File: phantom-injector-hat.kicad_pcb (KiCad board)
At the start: 2 copper layers, 65 x 44.8 mm, 42 parts, among them J1 Conn_02x20_Odd_Even, J2 Conn_02x03_Top_Bottom, J3 Conn_01x03, J4 Conn_01x03, SW1 SW_SPST, U1 LT8362EMSE-PBF

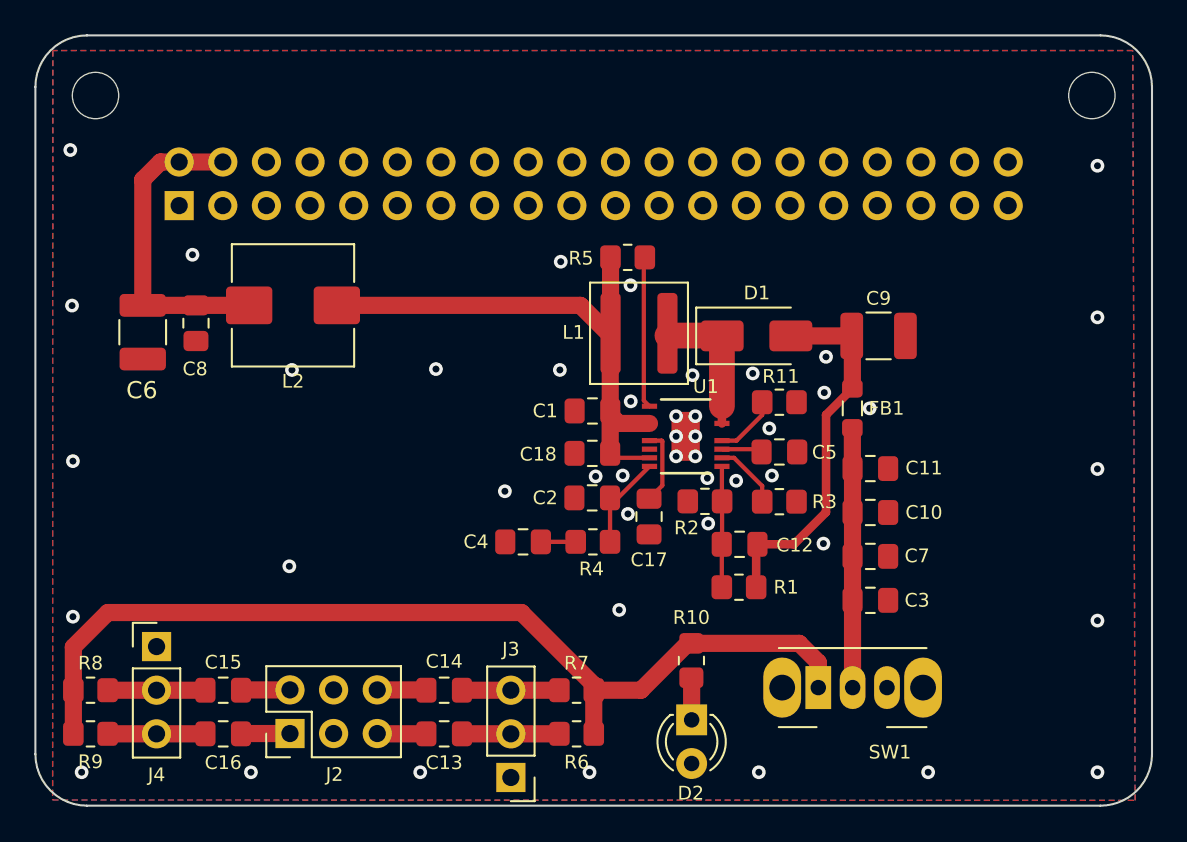
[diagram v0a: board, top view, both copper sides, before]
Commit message: Hopefully correct locations.
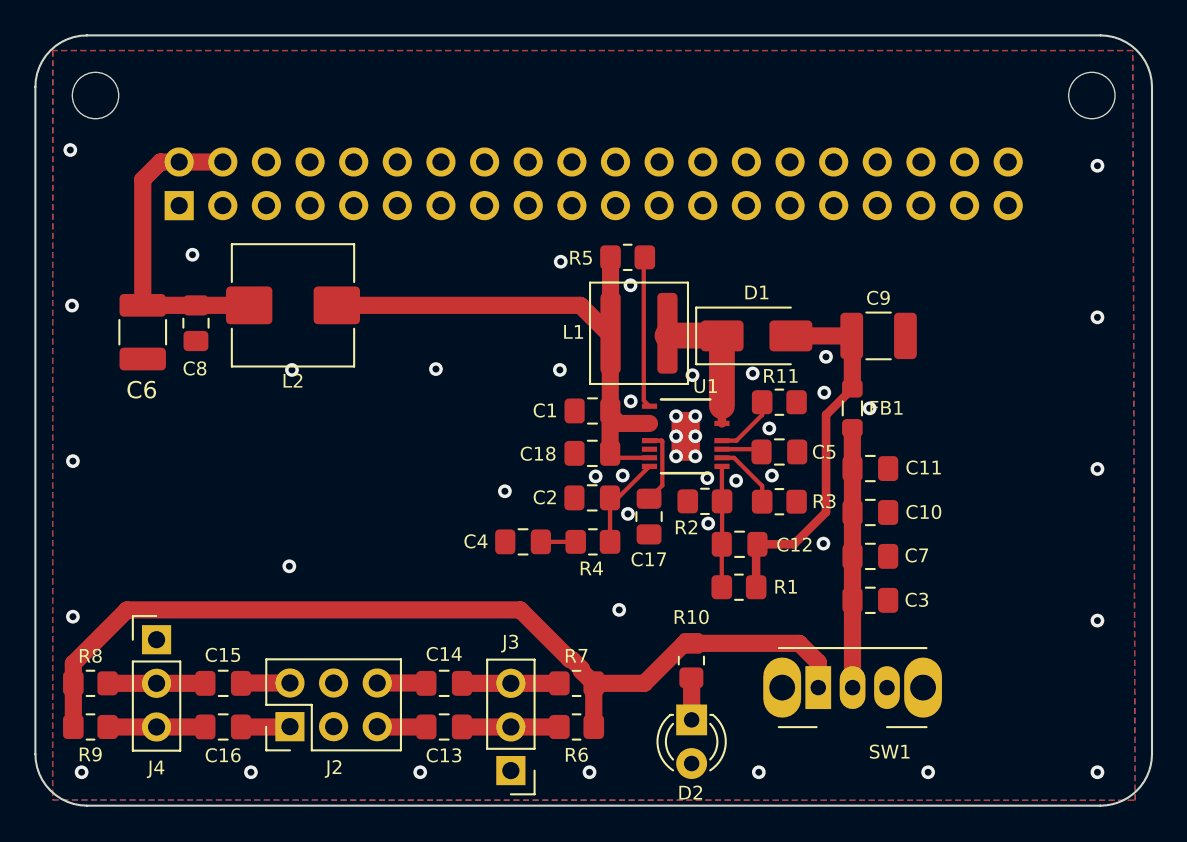
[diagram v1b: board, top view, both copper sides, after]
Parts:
- moved C13 0.40 mm to (123.8, 84.3)
- moved C16 0.40 mm to (110.9, 84.3)
- moved J2 0.40 mm to (114.8, 84.2)
- moved J3 0.40 mm to (127.7, 86.8)
- moved J4 0.40 mm to (107.1, 79.2)
- moved R6 0.40 mm to (131.5, 84.3)
- moved R9 0.40 mm to (103.2, 84.3)
- moved C14 0.40 mm to (123.8, 81.7)
- moved C15 0.40 mm to (110.9, 81.7)
- moved R7 0.40 mm to (131.5, 81.7)
- moved R8 0.40 mm to (103.2, 81.7)
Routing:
- net /+48V_SW: track 56.7 -> 55.6 mm
